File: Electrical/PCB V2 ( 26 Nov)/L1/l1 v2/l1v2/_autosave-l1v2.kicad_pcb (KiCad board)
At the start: 2 copper layers, 177.9 x 169.6 mm, 220 parts, among them J1 Conn_01x01_Socket, J2 Conn_01x01_Socket, SW1 SW_SPDT, U1 102010428, U2 CD74HC4067SM, U3 CD74HC4067SM

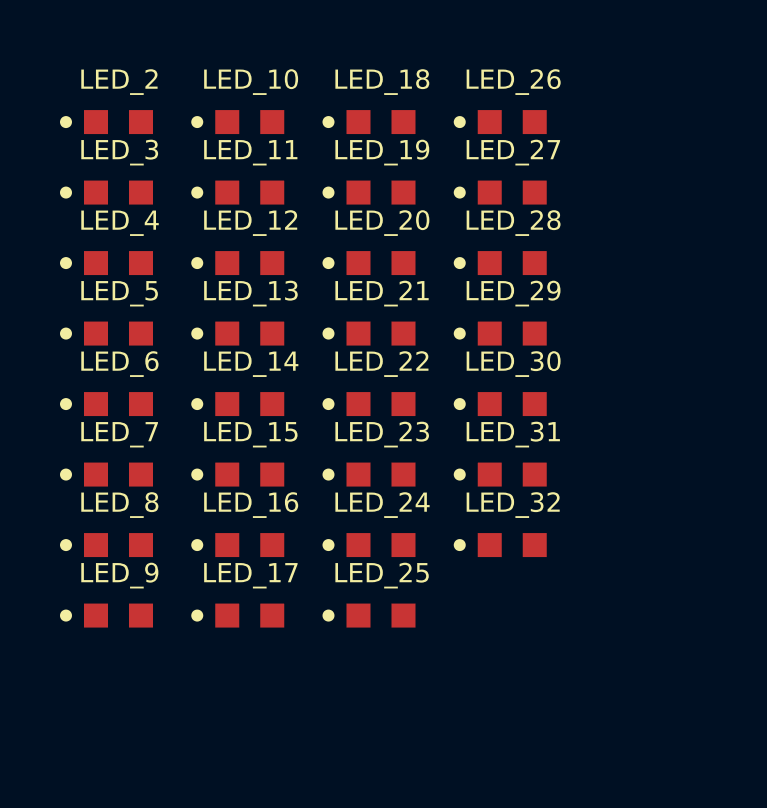
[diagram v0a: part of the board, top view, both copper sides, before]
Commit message: c
s
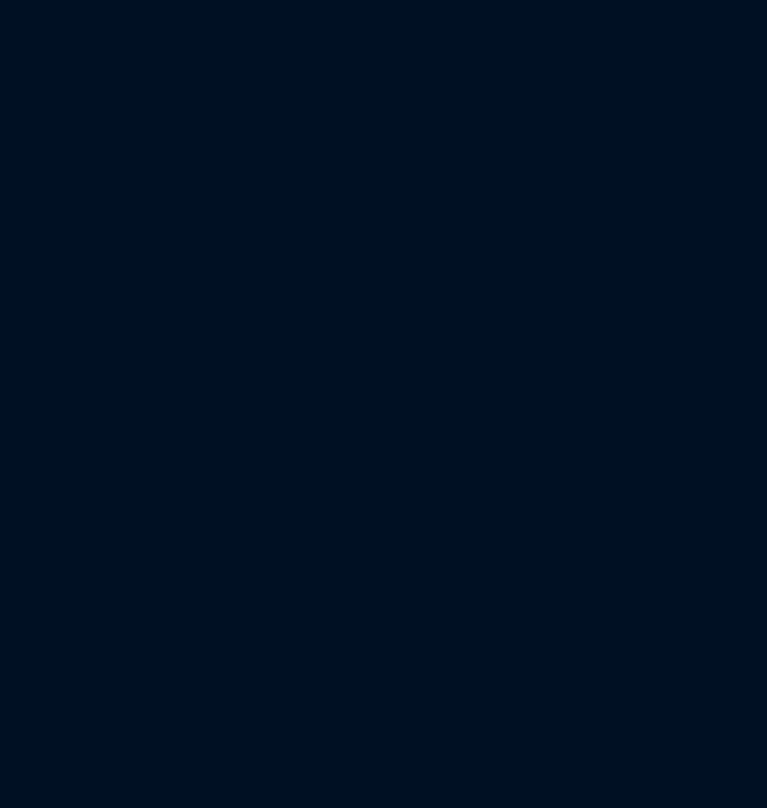
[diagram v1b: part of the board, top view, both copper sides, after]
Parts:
- removed LED_10, LED_11, LED_12, LED_13, LED_14, LED_15, LED_16, LED_17, LED_18, LED_19, LED_2, LED_20, LED_21, LED_22, LED_23, LED_24, LED_25, LED_26, LED_27, LED_28, LED_29, LED_3, LED_30, LED_31, LED_32, LED_4, LED_5, LED_6, LED_7, LED_8, LED_9: R_Photo, photoresistor:XDCR_ALS-PT19-315C_L177_TR8
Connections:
- LED_1 pad 1: 3v3 -> Net-(LED_1-Pad1)
